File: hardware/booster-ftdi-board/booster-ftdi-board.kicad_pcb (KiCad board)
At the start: 2 copper layers, 42.2 x 19.8 mm, 25 parts, among them J1 USB-B1HSB6, Q1 T2N7002AK, U1 FT231XS, U2 IF E96-E, U3 IF D95-T, U4 SN74LV1T34DBV, U5 SN74LV1T34DBV

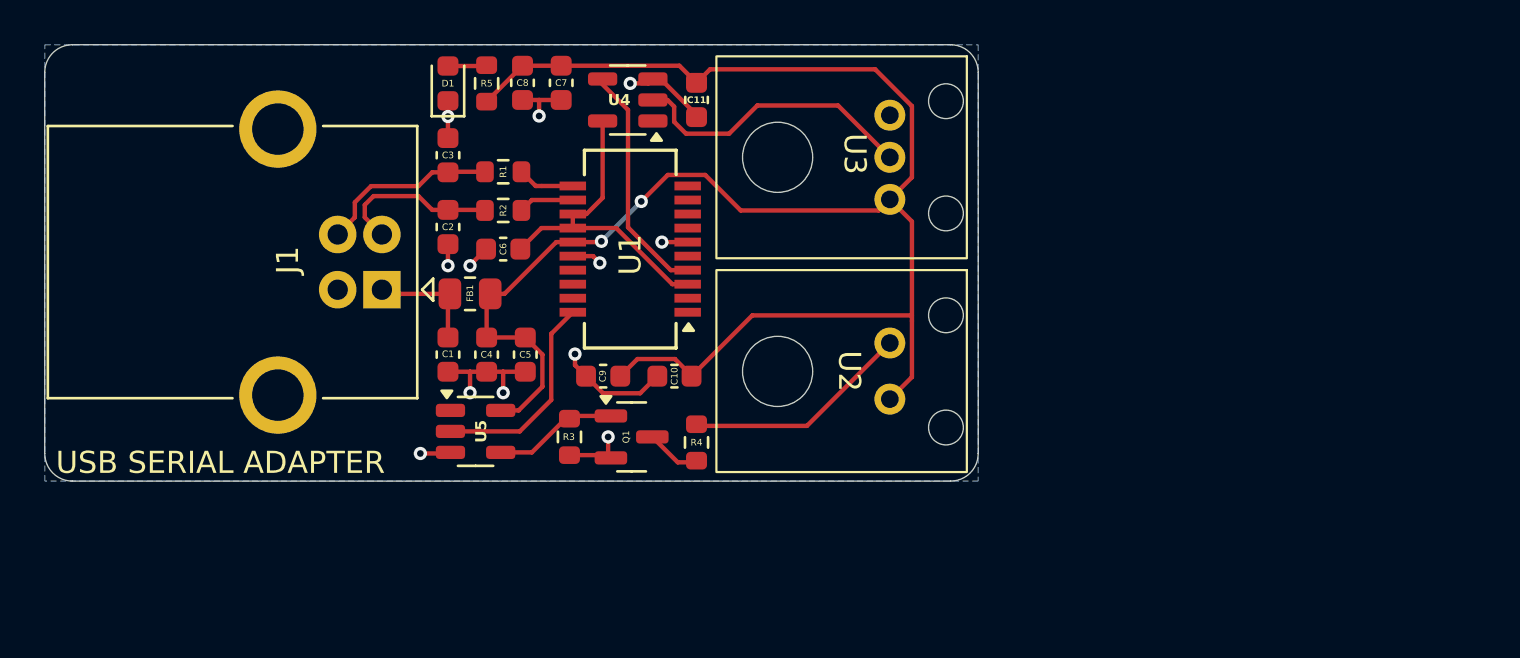
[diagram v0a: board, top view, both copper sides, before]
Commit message: v2 work
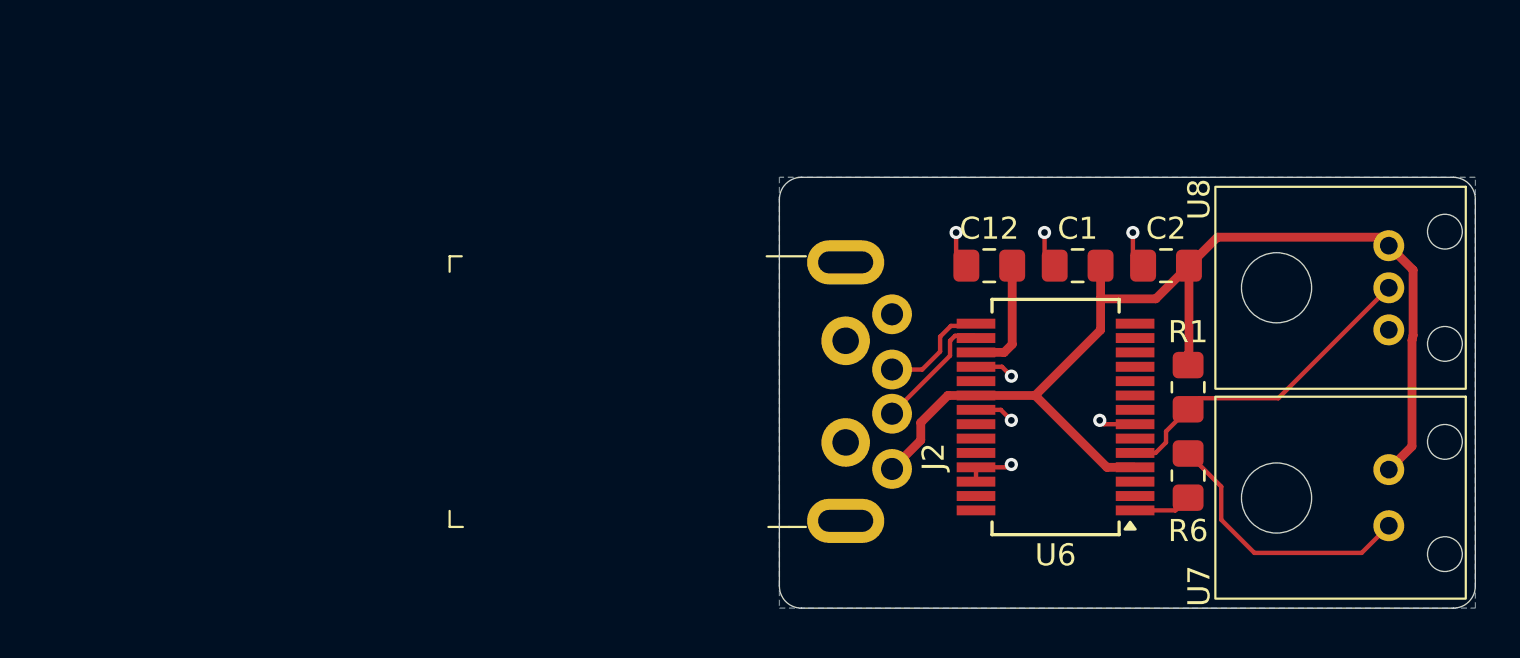
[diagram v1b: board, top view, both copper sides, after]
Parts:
- removed C10, C11, C4, C6, C7: 100n, Capacitor_SMD:C_0603_1608Metric
- removed C3: 47p, Capacitor_SMD:C_0603_1608Metric
- removed C5, C8, C9: 4u7, Capacitor_SMD:C_0603_1608Metric
- removed D1: 150060AS75000, LED_SMD:LED_0603_1608Metric
- removed FB1: MI0805K400R-10, Resistor_SMD:R_0805_2012Metric
- removed J1: USB-B1HSB6, Library:USB_B_OST_USB-B1HSxx_Horizontal
- removed Q1: T2N7002AK, Package_TO_SOT_SMD:SOT-23
- removed R2: 27R, Resistor_SMD:R_0603_1608Metric
- removed R3: 1k, Resistor_SMD:R_0603_1608Metric
- removed R4, R5: 150R, Resistor_SMD:R_0603_1608Metric
- removed U1: FT231XS, Package_SO:SSOP-20_3.9x8.7mm_P0.635mm
- removed U2: IF E96-E, Library:IF-E96E
- removed U3: IF D95-T, Library:IF-D95
- removed U4, U5: SN74LV1T34DBV, Package_TO_SOT_SMD:SOT-23-5
- added C12: 100n, Capacitor_SMD:C_0805_2012Metric_Pad1.18x1.45mm_HandSolder, F.Cu at (66.5, 32.5)
- added J2: UP2-AH-1-TH, digikey-footprints:USB_Male_A_UP2-AH-1-TH, F.Cu at (60.0, 38.2)
- added R6: 150R, Resistor_SMD:R_0805_2012Metric_Pad1.20x1.40mm_HandSolder, F.Cu at (75.5, 42.0)
- added U6: FT232RL, Package_SO:SSOP-28_5.3x10.2mm_P0.65mm, F.Cu at (69.5, 39.4)
- added U7: IF E96-E, Library:IF-E96E, F.Cu at (88.1, 39.5)
- added U8: IF D95-T, Library:IF-D95, F.Cu at (88.1, 30.0)
- C1: value 10n -> 4u7; footprint Capacitor_SMD:C_0603_1608Metric -> Capacitor_SMD:C_0805_2012Metric_Pad1.18x1.45mm_HandSolder
- C2: value 47p -> 100n; footprint Capacitor_SMD:C_0603_1608Metric -> Capacitor_SMD:C_0805_2012Metric_Pad1.18x1.45mm_HandSolder
- R1: value 27R -> 10k; footprint Resistor_SMD:R_0603_1608Metric -> Resistor_SMD:R_0805_2012Metric_Pad1.20x1.40mm_HandSolder
- moved C2 32.5 mm to (74.5, 32.5), turned to 0 degrees
- moved R1 32.5 mm to (75.5, 38.0), turned to -90 degrees
- moved C1 28.8 mm to (70.5, 32.5), turned to 0 degrees
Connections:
- C1 pad 2: Net-(J1-VBUS) -> VCC
- C2 pad 1: /USBI_N -> GND
- C2 pad 2: GND -> VCC
- R1 pad 1: /USBI_P -> VCC
- R1 pad 2: /USB_P -> Net-(U6-RXD)
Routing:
- net VCC: track 80.9 -> 51.2 mm, vias 2 -> 0
- net +3V3: track 15.0 -> 0.00 mm
- net GND: track 27.5 -> 12.6 mm, vias 12 -> 7
- net Net-(U6-RXD): track 0.00 -> 14.9 mm
- net Net-(U3-OUT): track 13.6 -> 0.00 mm
- net Net-(U7-K): track 0.00 -> 12.3 mm
- net Net-(U1-RXD): track 10.8 -> 0.00 mm
- net Net-(U2-K): track 10.3 -> 0.00 mm
- net Net-(U1-TXD): track 9.52 -> 0.00 mm
- net /USBI_P: track 8.20 -> 0.00 mm
- net /USBI_N: track 7.50 -> 0.00 mm
- net Net-(Q1-G): track 6.04 -> 0.00 mm
- net /USB_-: track 0.00 -> 5.70 mm
- net Net-(U6-3V3OUT): track 0.00 -> 5.50 mm
- net Net-(J1-VBUS): track 5.16 -> 0.00 mm
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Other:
- board size 42.2 x 19.8 mm -> 31.5 x 19.5 mm
- board text removed: "USB SERIAL ADAPTER"
